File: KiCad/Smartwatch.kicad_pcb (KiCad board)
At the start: 4 copper layers, 38.5 x 38.5 mm, 96 parts, among them J1 5358, M1 LCM1027B3605F, Q1 AO3400A, SW1 SW_Push, SW2 JXTCONN TS-1010-S26, U1 BNO055, U10 Quectel LC76G, U11 MIC5504-1.8YM5, U12 ESP32-S3, U13 BMP280, U14 LD39100PU33R, U2 MIC5504-3.3YM5, U3 MAX30102, U4 MCP9808_DFN, U5 TPS2116DRL, U6 USBLC6-2SC6, U7 BRCL4054DME, U9 GC9A01_IPS_Display_w/_Touch, Y1 40MHz, Y2 32.768KHz, Y3 32.768KHz

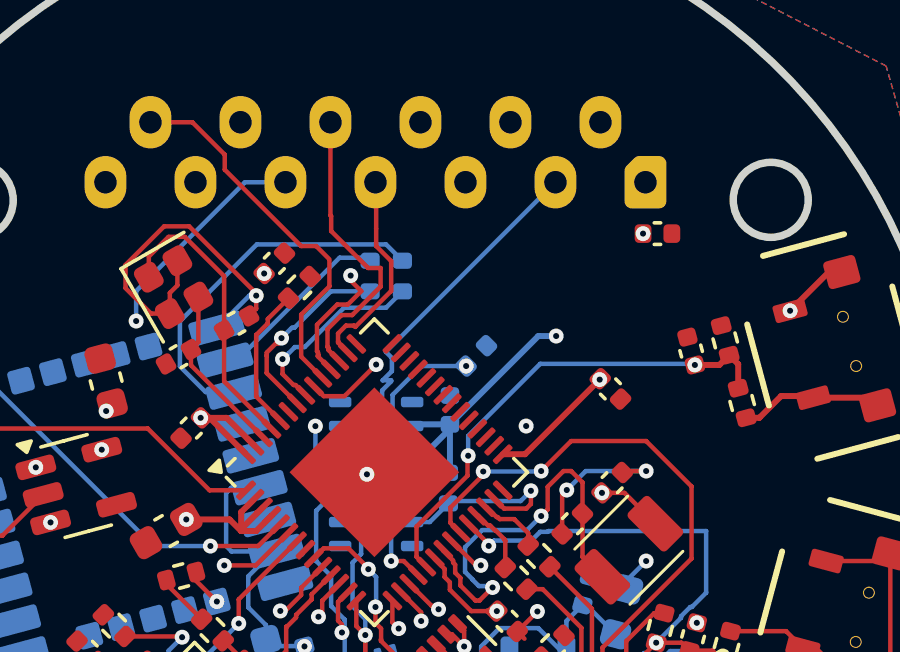
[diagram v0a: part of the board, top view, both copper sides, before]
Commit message: minor updates - practice pulling to local branch
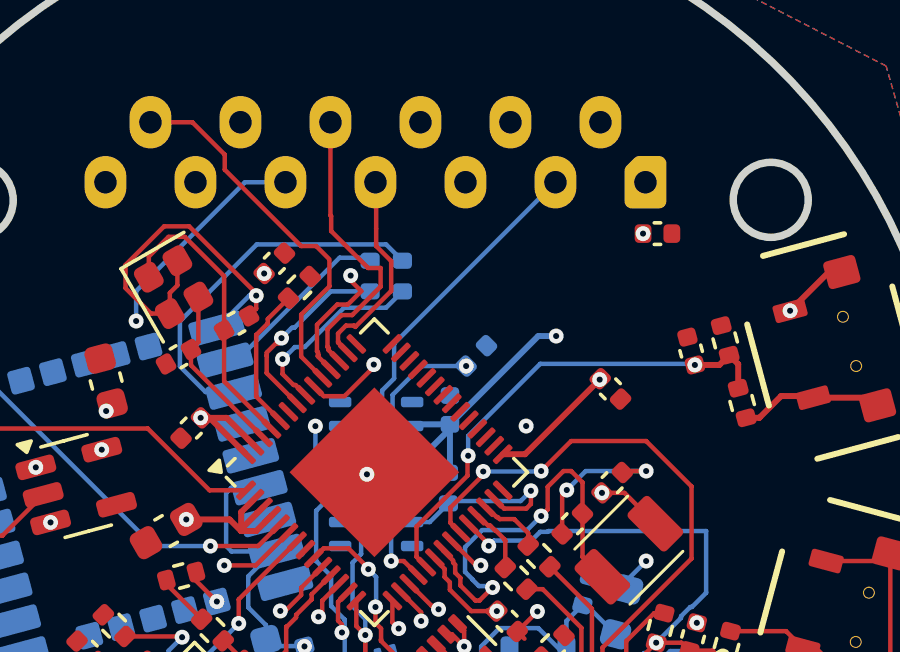
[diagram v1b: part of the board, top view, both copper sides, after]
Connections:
- C19 pad 1: Net-(U1-CAP) -> GND
- C19 pad 2: GND -> Net-(U1-CAP)
- R21 pad 1: GND -> Net-(U1-PS0)
- R21 pad 2: Net-(U1-PS0) -> GND
- R22 pad 1: GND -> Net-(U1-PS1)
- R22 pad 2: Net-(U1-PS1) -> GND
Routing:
- net /CS: track 25.4 -> 22.1 mm
- net /MISO: track 16.8 -> 16.2 mm
